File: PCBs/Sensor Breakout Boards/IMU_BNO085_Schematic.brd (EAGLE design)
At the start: 25.4 x 25.4 mm, 8 parts, among them J1 2X6 FEMALE

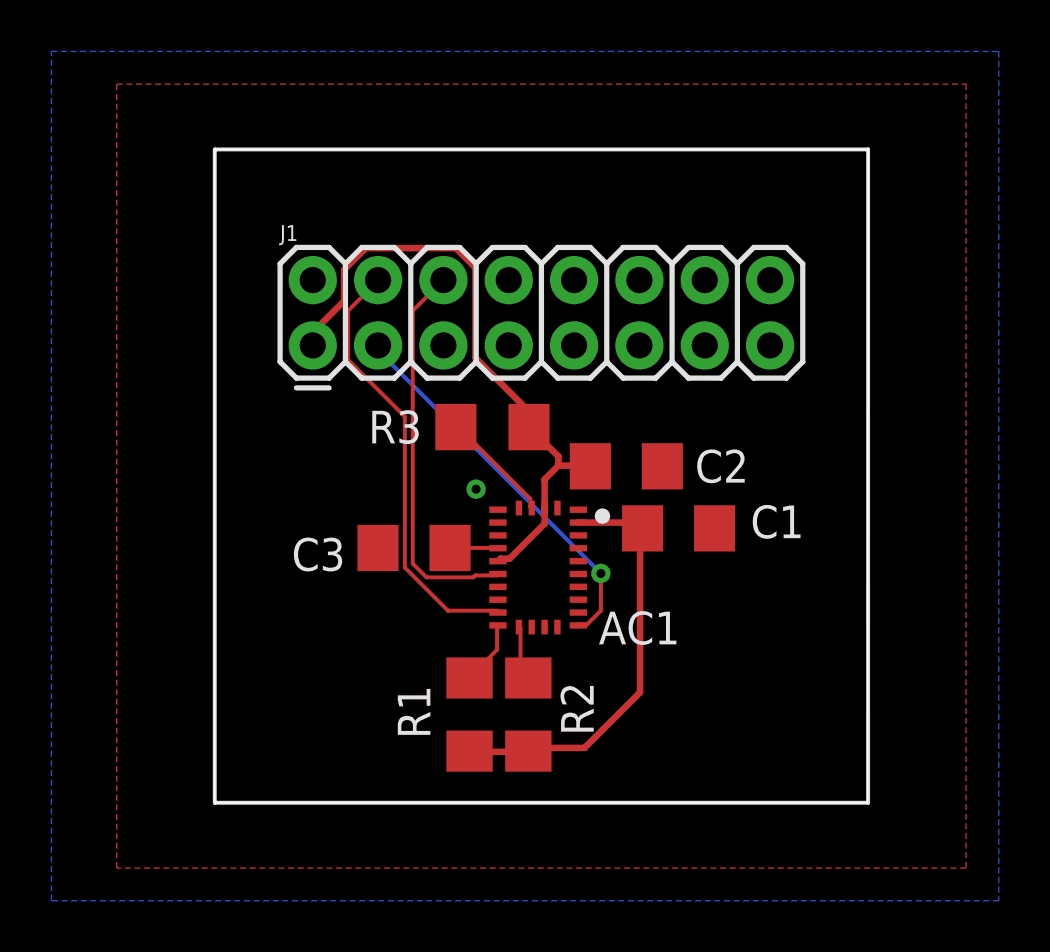
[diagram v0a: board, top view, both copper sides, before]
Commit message: Prep for JLC?
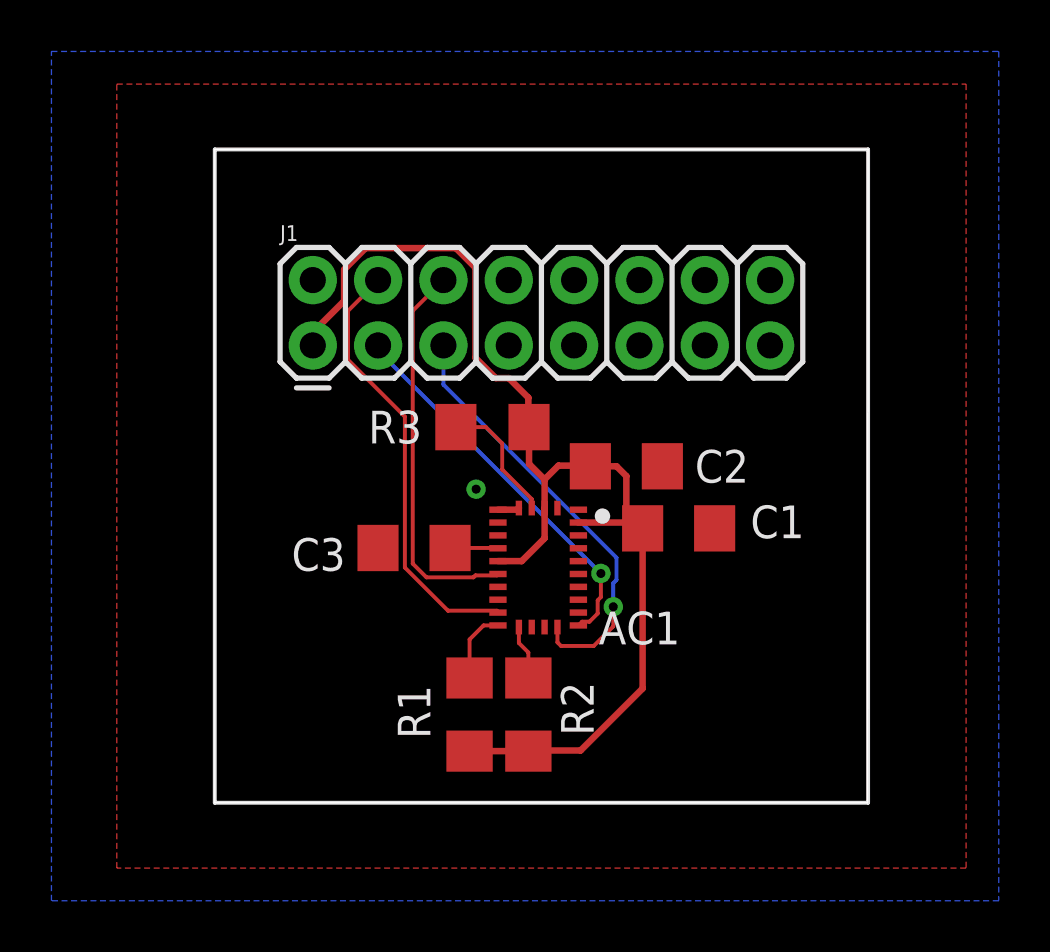
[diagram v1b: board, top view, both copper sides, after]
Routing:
- net SCL: track 0.00 -> 16.9 mm, vias 0 -> 1
- net VCC: track 41.3 -> 45.8 mm
- net GND: track 0.00 -> 0.84 mm, vias 0 -> 1
- net N$8: track 4.45 -> 5.05 mm
